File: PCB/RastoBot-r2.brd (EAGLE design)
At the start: 200 x 130 mm, 354 parts, among them IC1 PIC24FJ32GA002-X, Q1 FDD4141TO252, Q8 FDD4141TO252, T2 2N2222A, U1 PIC18F47J13-I/PT, U10 140357145000, U11 140357145000, U12 140357145000, U13 140357145000, U15 PIC32MK1024MCM064-I/PTTQFP64_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, U2 LIS3MDLTR, U4 140357145000, U5 MPU-6050, U6 140357145000, U7 140357145000, U8 140357145000, U9 140357145000, X5 FPS009-3000

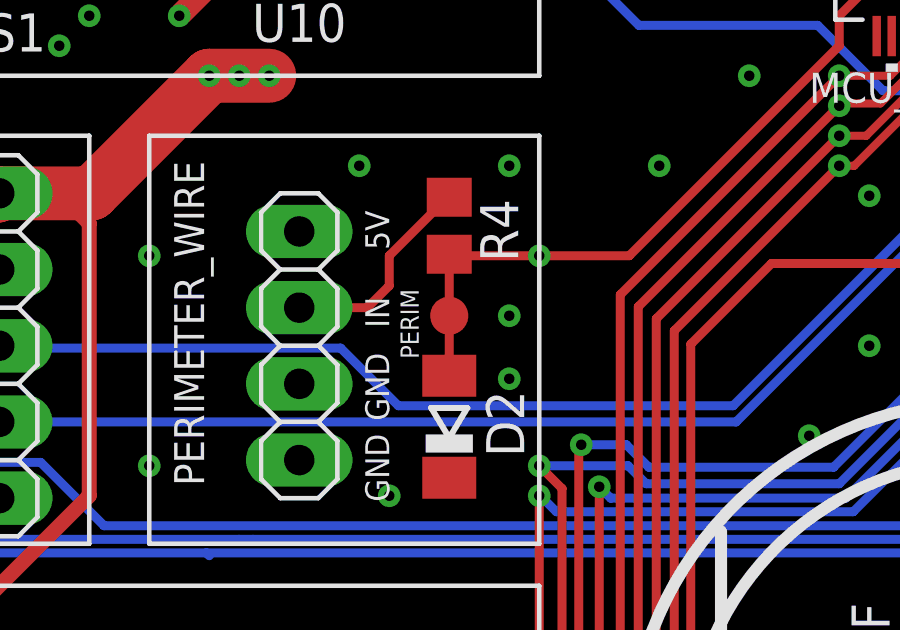
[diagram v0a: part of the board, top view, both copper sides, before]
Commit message: GPS
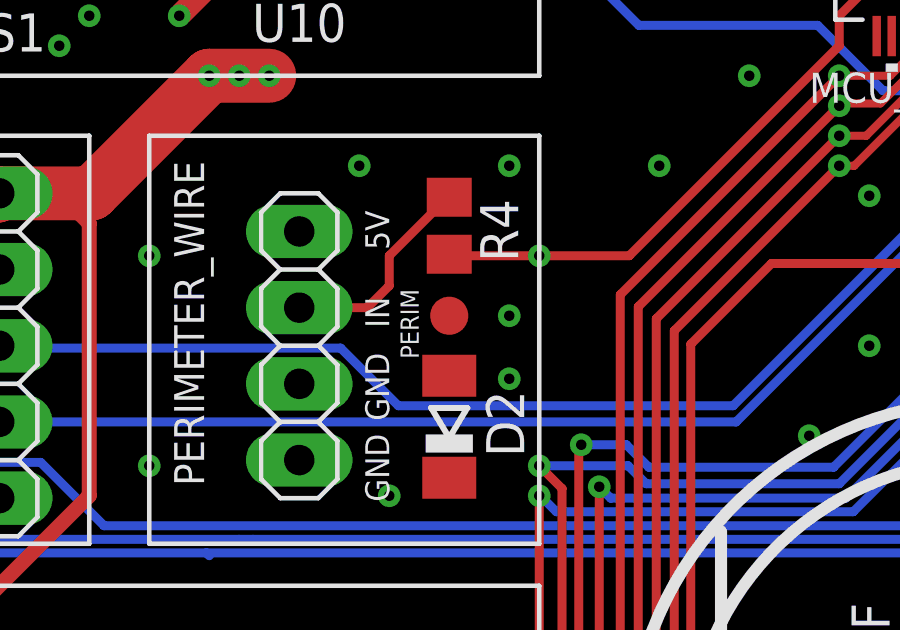
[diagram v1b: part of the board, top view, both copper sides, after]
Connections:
- net GND: now also D2.A; no longer D2.C
- net PERIMETER_WIRE_SENSE: now also D2.C; no longer D2.A
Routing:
- net PERIMETER_WIRE_SENSE: track 34.8 -> 28.7 mm
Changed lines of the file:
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@@
 <contactref element="PERIMETER_WIRE" pad="4"/>
 <contactref element="PERIMETER_WIRE" pad="3"/>
-<contactref element="D2" pad="C"/>
 <contactref element="LIMIT_SWITCH_UP" pad="3"/>
 <contactref element="R110" pad="1"/>
@@
 <contactref element="MCU_2_I2C_EXTENDER" pad="4"/>
 <contactref element="U5" pad="1"/>
+<contactref element="D2" pad="A"/>
 <wire x1="145.15" y1="110" x2="141.85" y2="112" width="0" layer="19" extent="1-1"/>
 <wire x1="146" y1="107.85" x2="145.15" y2="110" width="0" layer="19" extent="1-1"/>
@@
 <wire x1="119" y1="34" x2="119" y2="39" width="0" layer="19" extent="1-1"/>
 <wire x1="119" y1="31.9" x2="119" y2="34" width="0" layer="19" extent="1-1"/>
-<wire x1="117" y1="28.6" x2="119" y2="31.9" width="0" layer="19" extent="1-1"/>
-<wire x1="115" y1="28" x2="117" y2="28.6" width="0" layer="19" extent="1-1"/>
+<wire x1="117" y1="32" x2="119" y2="31.9" width="0" layer="19" extent="1-1"/>
+<wire x1="115" y1="28" x2="117" y2="32" width="0" layer="19" extent="1-1"/>
 <wire x1="112" y1="29.19" x2="115" y2="28" width="0" layer="19" extent="1-1"/>
 <wire x1="112" y1="31.73" x2="112" y2="29.19" width="0" layer="19" extent="1-1"/>
@@
 </signal>
 <signal name="PERIMETER_WIRE_SENSE">
-<contactref element="R4" pad="1"/>
-<contactref element="D2" pad="A"/>
 <contactref element="U15" pad="4"/>
-<wire x1="117" y1="36.05" x2="117" y2="32" width="0.3" layer="1"/>
-<wire x1="117" y1="36.05" x2="117.05" y2="36" width="0.3" layer="1"/>
 <wire x1="117.05" y1="36" x2="120" y2="36" width="0.3" layer="1"/>
 <via x="120" y="36" extent="1-16" drill="0.35"/>
@@
 <wire x1="137.6706" y1="45.6706" x2="138.75" y2="46.75" width="0.28" layer="1"/>
 <contactref element="PERIM" pad="TP"/>
-<wire x1="117" y1="34" x2="117" y2="32" width="0.1524" layer="1"/>
+<contactref element="D2" pad="C"/>
+<contactref element="R4" pad="1"/>
+<wire x1="117" y1="36.05" x2="117.05" y2="36" width="0" layer="19" extent="1-1"/>
+<wire x1="117" y1="34" x2="117.05" y2="36" width="0" layer="19" extent="1-1"/>
+<wire x1="117" y1="28.6" x2="117" y2="34" width="0" layer="19" extent="1-1"/>
 </signal>
 <signal name="N$79">
